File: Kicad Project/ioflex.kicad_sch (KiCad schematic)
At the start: 2 parts, among them CN12 DF40C-50DS-0.4V, CN13 DF40C-50DS-0.4V

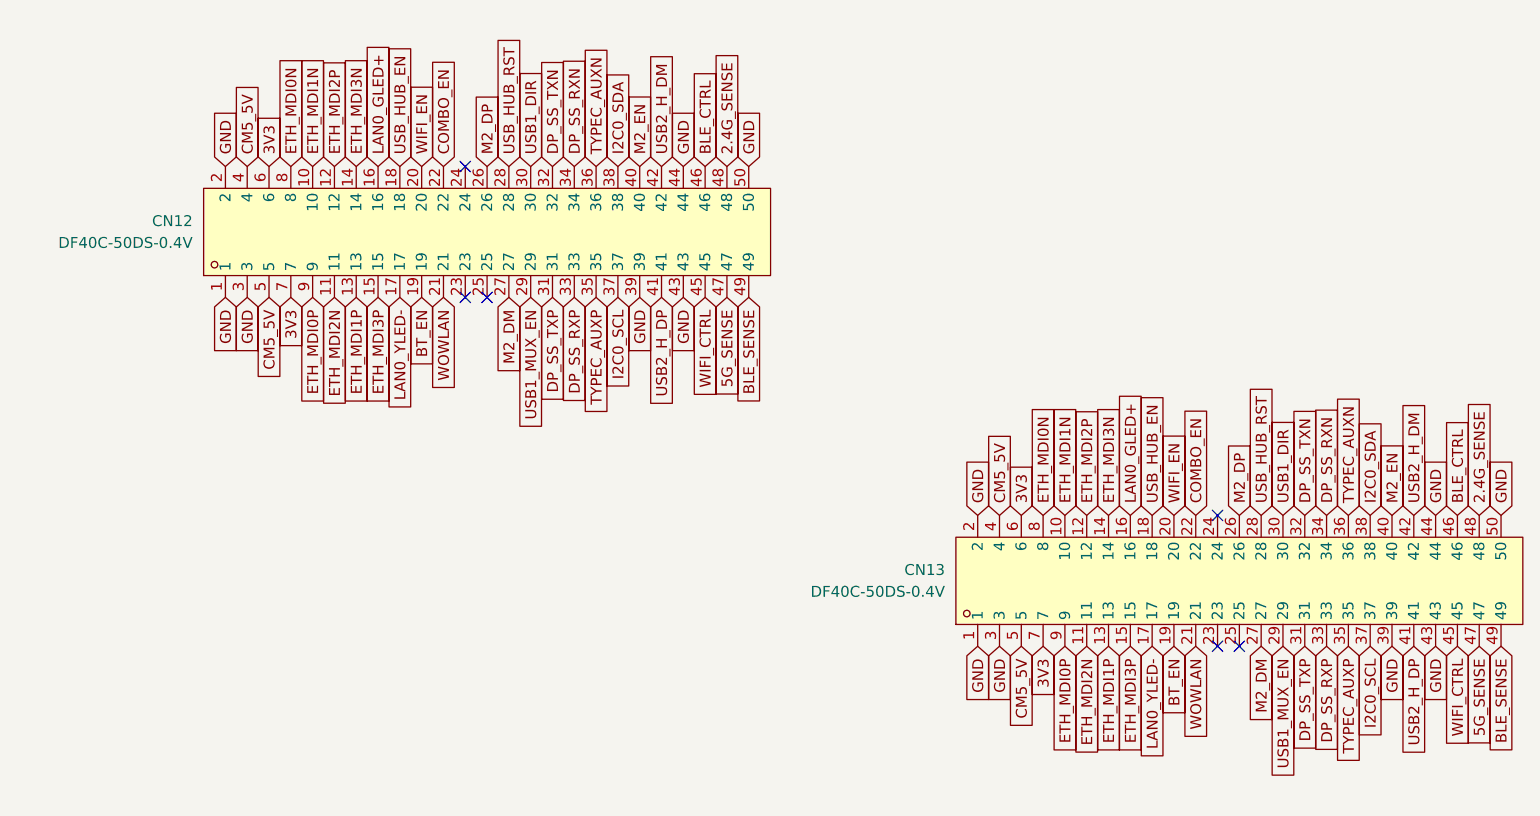
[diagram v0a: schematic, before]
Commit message: made some schematic changes to power
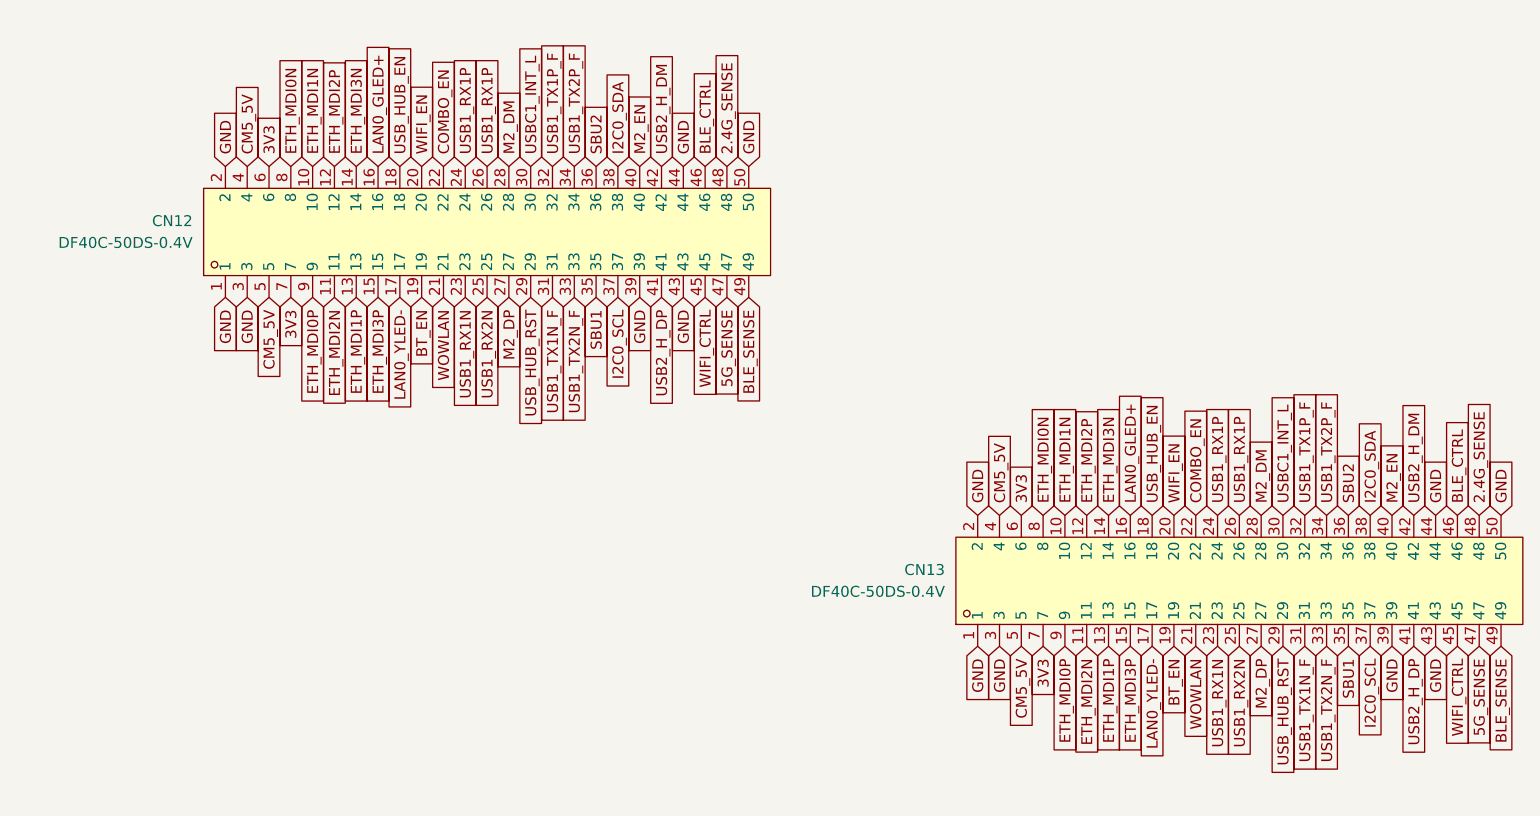
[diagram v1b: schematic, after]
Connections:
- net USB1_MUX_EN is gone; now on net USB_HUB_RST: CN12.29, CN13.29
- net M2_DM: now also CN12.28, CN13.28; no longer CN12.27, CN13.27
- net M2_DP: now also CN12.27, CN13.27; no longer CN12.26, CN13.26
- net USB_HUB_RST: no longer CN12.28, CN13.28
- net USB1_RX1N: now reaches CN13.23
- net USB1_RX1N: now also CN12.23
- net USB1_RX1P: now reaches CN13.24
- net USB1_RX1P: now also CN12.24, CN12.26, CN13.26
- net USB1_RX2N: now reaches CN13.25
- net USB1_RX2N: now also CN12.25
- net DP_SS_RXN renamed USB1_TX2P_F
- net DP_SS_RXP renamed USB1_TX2N_F
- net DP_SS_TXN renamed USB1_TX1P_F
- net DP_SS_TXP renamed USB1_TX1N_F
- net TYPEC_AUXN renamed SBU2
- net TYPEC_AUXP renamed SBU1
- net USB1_DIR renamed USBC1_INT_L
- no-connect marks 6 -> 0
